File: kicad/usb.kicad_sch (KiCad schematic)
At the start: 3 parts, among them J5 USB4145-03-0230-C

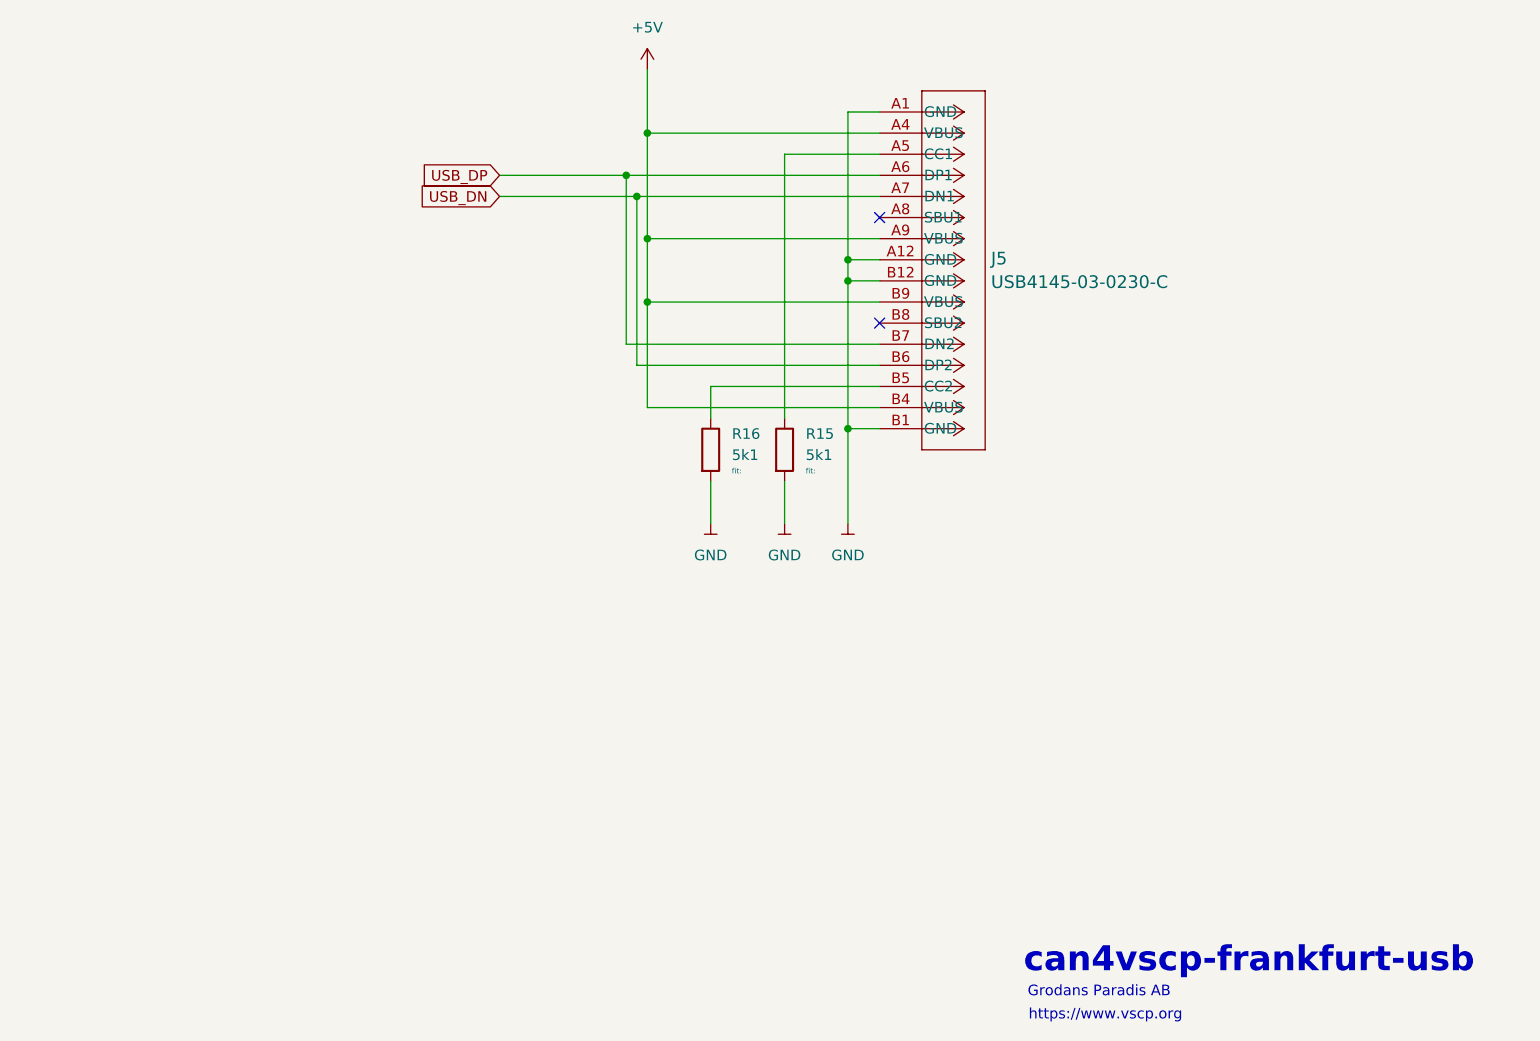
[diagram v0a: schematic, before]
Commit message: Reversion A schema and PCB
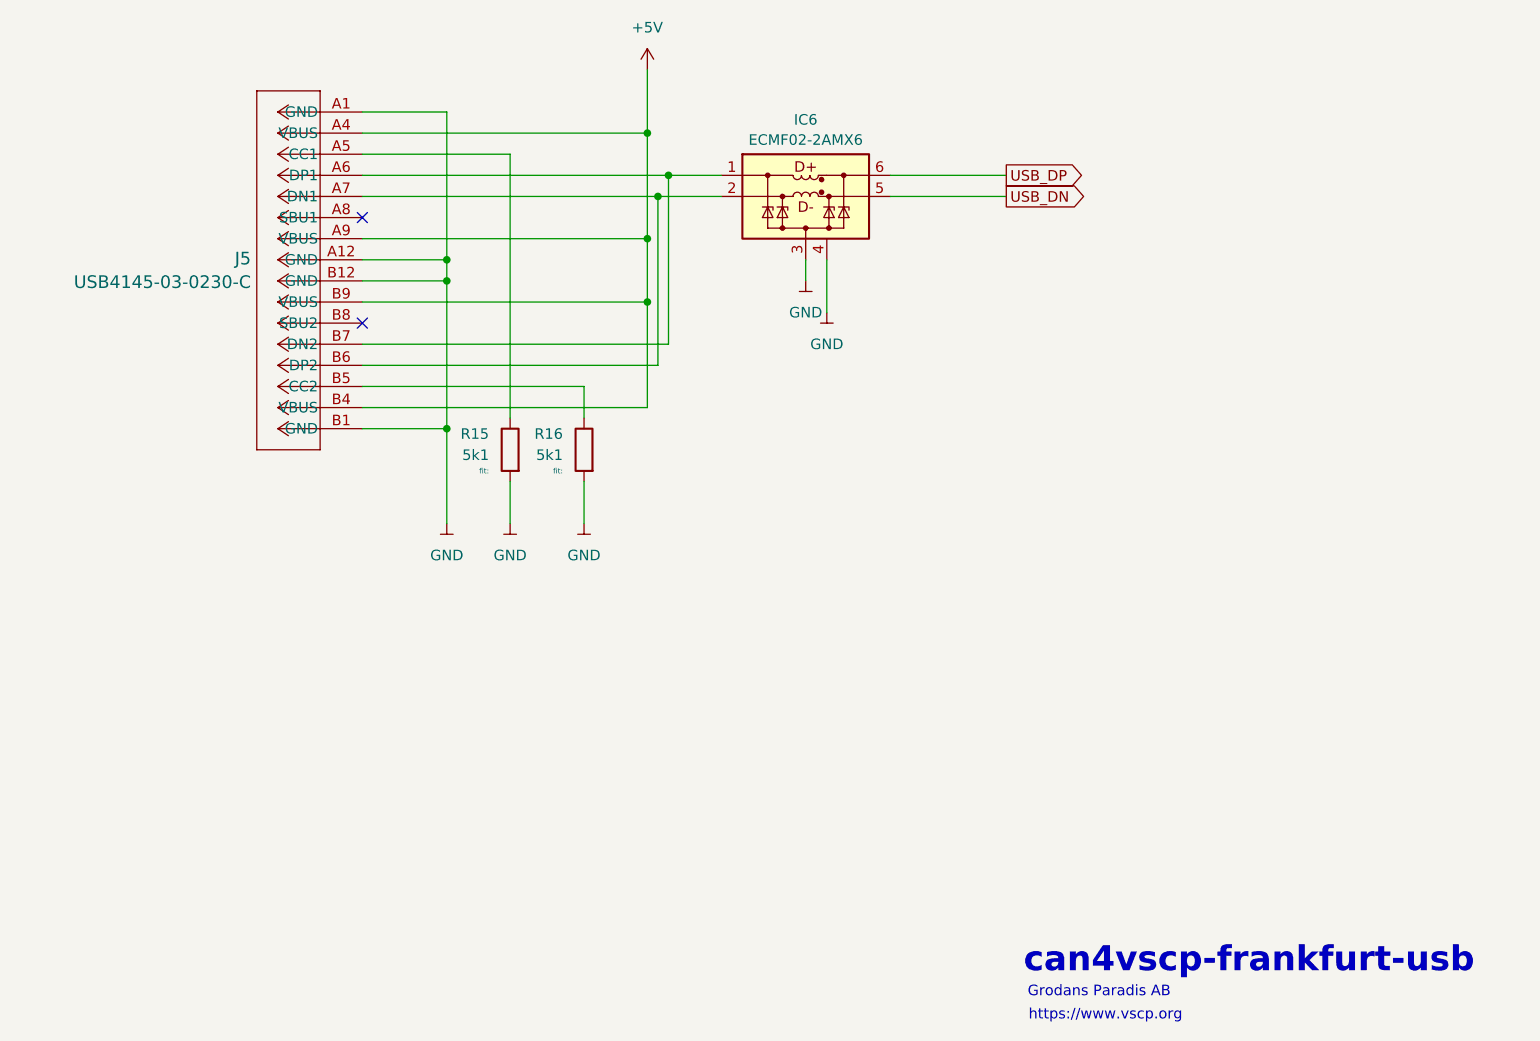
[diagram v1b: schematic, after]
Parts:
- added IC6: ECMF02-2AMX6, Package_DFN_QFN:ST_UQFN-6L_1.5x1.7mm_P0.5mm, symbol Power_Protection:ECMF02-2AMX6
- J5: footprint CONN_USB4145-03-0230-C_GCT -> USB4145-03-0230-C:CONN_USB4145-03-0230-C_GCT
- R15, R16: footprint Resistors_SMD:R_0603 -> Resistor_SMD:R_0805_2012Metric
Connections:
- net GND: now also IC6.3 (GND), IC6.4 (NC)
- net USB_DN: now also IC6.5 (D-_out); no longer J5.A7 (DN1), J5.B6 (DP2)
- net USB_DP: now also IC6.6 (D+_out); no longer J5.A6 (DP1), J5.B7 (DN2)
- new net: IC6.1 (D+_in), J5.A6 (DP1), J5.B7 (DN2)
- new net: IC6.2 (D-_in), J5.A7 (DN1), J5.B6 (DP2)
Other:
- moved on the sheet: J5, R15, R16
